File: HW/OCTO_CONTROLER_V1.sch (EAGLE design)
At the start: 58 parts, among them IC1 CXDM4060P, IC2 AOZ1284PI, J1 DC_POWER, Q1 CXDM4060P, Q10 DTDG23YP, Q2 CXDM4060P, Q3 DTC114EUA, Q4 DTC114EUA, Q5 DTC114EUA, Q6 DTC114EUA, Q7 DTC114EUA, Q8 DTC114EUA, Q9 DTDG23YP, X1 RASPI_BOARD_B+#_F

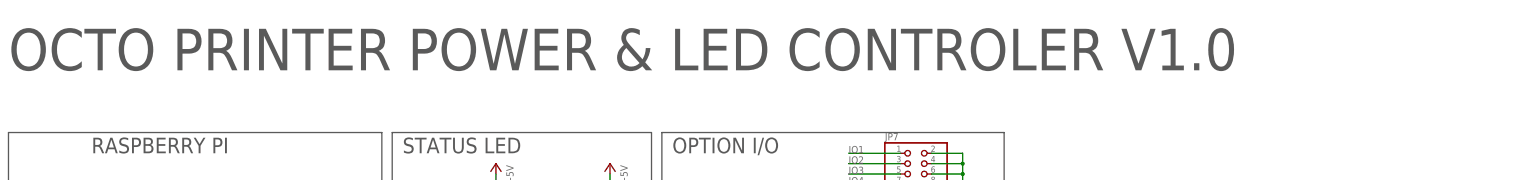
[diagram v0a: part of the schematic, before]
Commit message: RENAME PCB DESIGN FILE
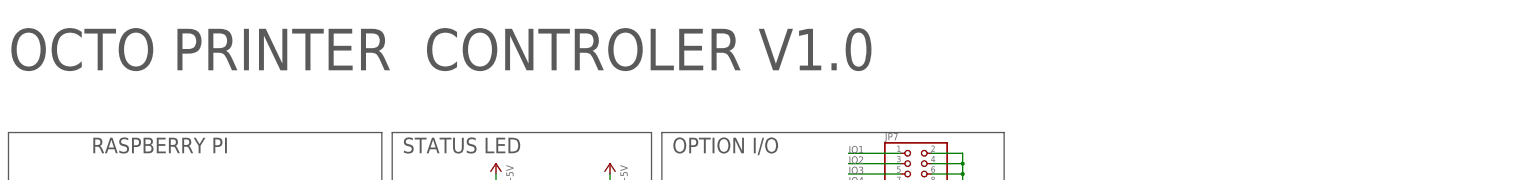
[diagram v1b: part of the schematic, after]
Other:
- note added: "OCTO PRINTER CONTROLER V1.0"
- note removed: "OCTO PRINTER POWER & LED CONTROLER V1.0"
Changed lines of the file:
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@@
 <sheet>
 <plain>
-<text x="-208.28" y="53.34" size="10.16" layer="97">OCTO PRINTER POWER &amp; LED CONTROLER V1.0</text>
+<text x="-208.28" y="53.34" size="10.16" layer="97">OCTO PRINTER  CONTROLER V1.0</text>
 <wire x1="-208.28" y1="-53.34" x2="-119.38" y2="-53.34" width="0.1524" layer="97"/>
 <wire x1="-208.28" y1="-144.78" x2="-119.38" y2="-144.78" width="0.1524" layer="97"/>
